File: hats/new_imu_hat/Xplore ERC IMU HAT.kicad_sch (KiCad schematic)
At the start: 32 parts, among them J1 BM08B-GHS-TBT, J2 5025850670, J3 BM04B-GHS-TBT, J4 Hat_connector_hole, J5 5025850670, SW1 SW_DIP_x01, U1 LT3960JMSE-PBF, U2 D5V0H1B2LP-7B

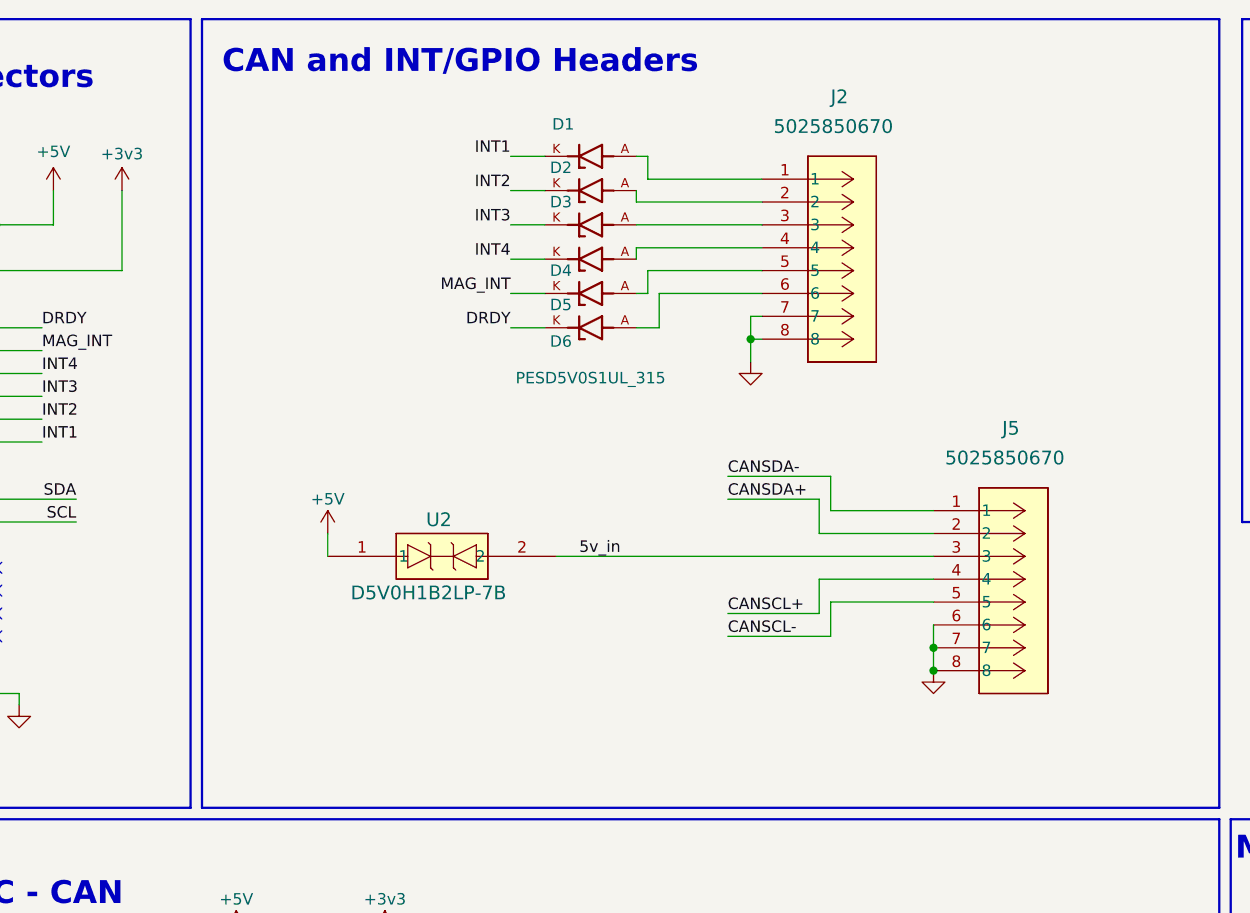
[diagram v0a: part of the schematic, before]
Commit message: IMU tweaks
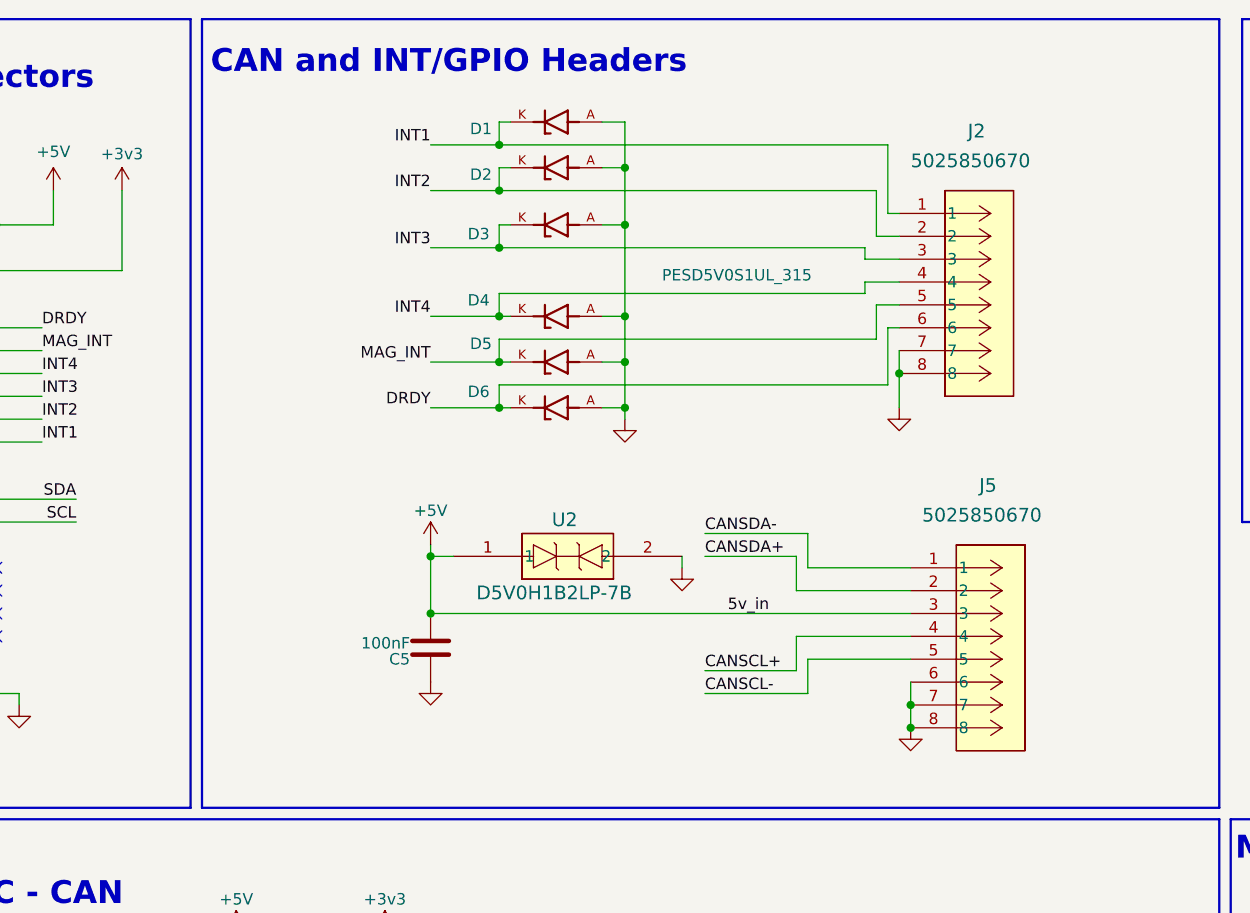
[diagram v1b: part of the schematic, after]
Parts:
- added C5: 100nF, Capacitor_SMD:C_0402_1005Metric, symbol Device:C
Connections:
- net +5V: now also J5.3, C5.2
- net DRDY: now also J2.6
- net GND: now also D1.A, D2.A, D3.A, D4.A, D5.A, D6.A, U2.2, C5.1
- net INT1: now also J2.1
- net INT2: now also J2.2
- net INT3: now also J2.3
- net INT4: now also J2.4
- net MAG_INT: now also J2.5
- removed net 5v_in: J5.3, U2.2
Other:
- moved on the sheet: J5
